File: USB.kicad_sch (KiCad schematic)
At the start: 39 parts, among them J1 PDM MEMS Mic, J2 24FLZ-SM2-TB, J5 DM3BT-DSF-PEJS, Q1 AO3401A, U3 FDS9926A

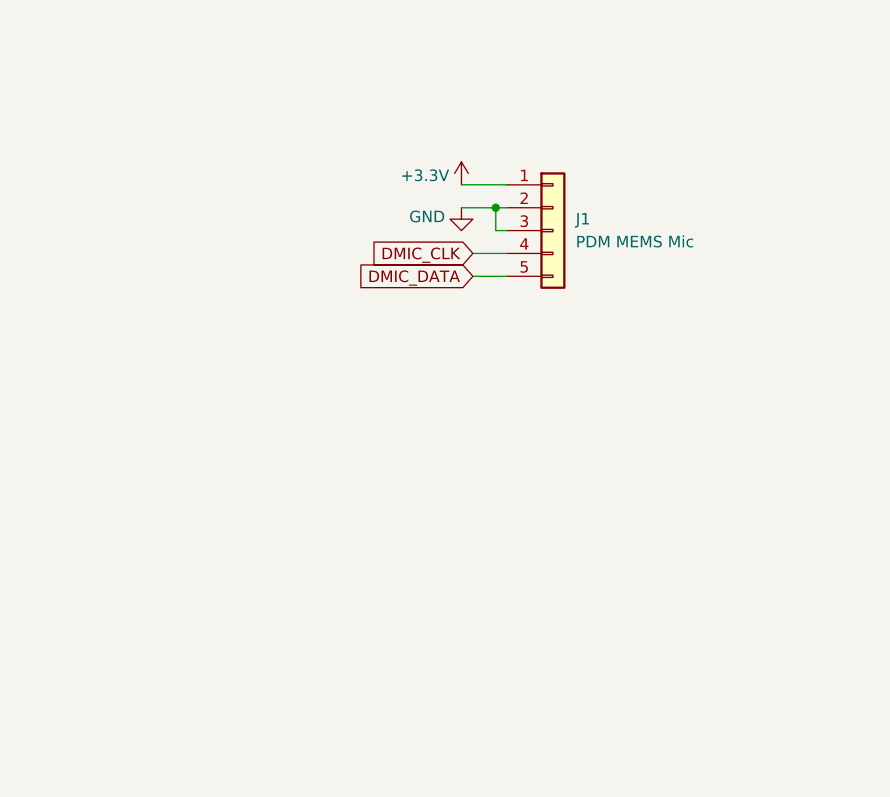
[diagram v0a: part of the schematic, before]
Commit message: I think I'm done. Fingers crossed.
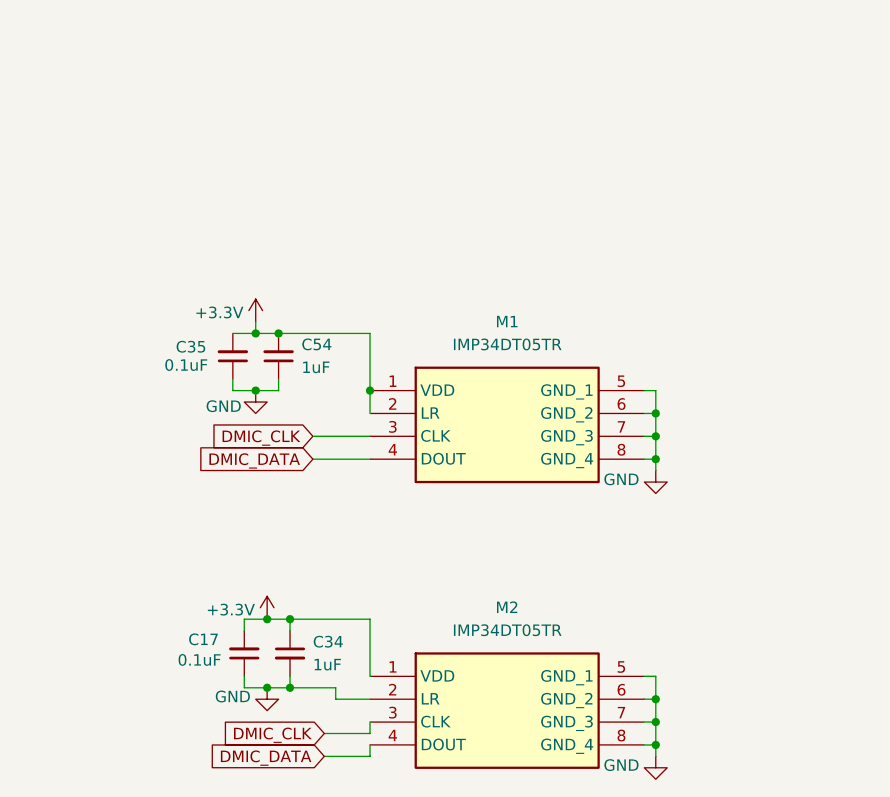
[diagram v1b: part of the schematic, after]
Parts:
- removed J1: PDM MEMS Mic, Adafruit:Adafruit MEMS 3492, symbol Connector_Generic:Conn_01x05
- added C17, C35: 0.1uF, Capacitor_SMD:C_0201_0603Metric_Pad0.64x0.40mm_HandSolder, symbol Device:C_Small
- added C34, C54: 1uF, Capacitor_SMD:C_0201_0603Metric_Pad0.64x0.40mm_HandSolder, symbol Device:C_Small
- added M1, M2: IMP34DT05TR, IMP34DT05TR, symbol IMP34DT05TR:IMP34DT05TR
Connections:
- net +3.3V: now also C17.2, C34.1, C35.2, C54.2, M1.1 (VDD), M1.2 (LR), M2.1 (VDD)
- net DMIC_CLK: now also M1.3 (CLK), M2.3 (CLK)
- net DMIC_DATA: now also M1.4 (DOUT), M2.4 (DOUT)
- net GND: now also C17.1, C34.2, C35.1, C54.1, M1.5 (GND_1), M1.6 (GND_2), M1.7 (GND_3), M1.8 (GND_4), M2.2 (LR), M2.5 (GND_1), M2.6 (GND_2), M2.7 (GND_3), M2.8 (GND_4)
